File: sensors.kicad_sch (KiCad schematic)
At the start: 0 parts

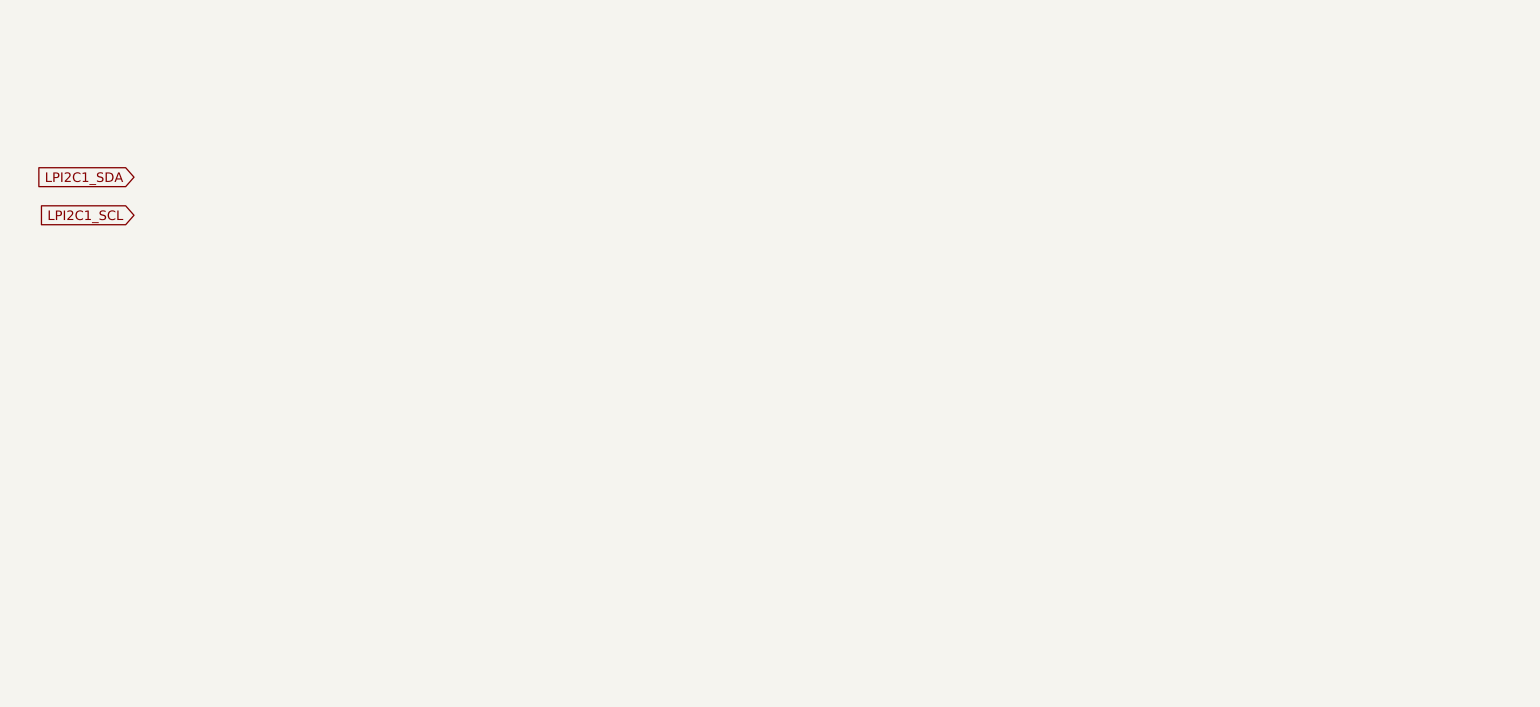
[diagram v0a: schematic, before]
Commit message: finished v1
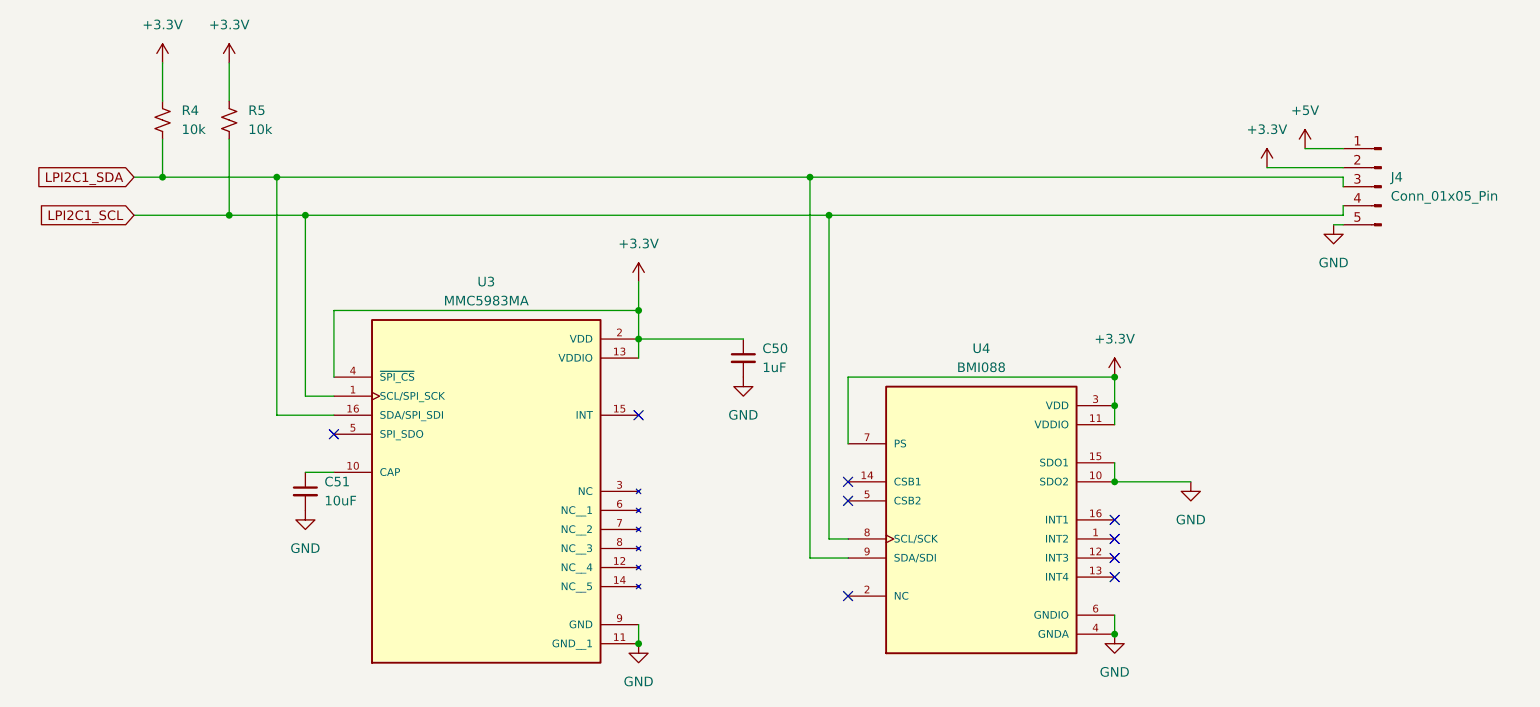
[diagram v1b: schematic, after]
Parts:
- added C50: 1uF, symbol Device:C_Small
- added C51: 10uF, symbol Device:C_Small
- added J4: Conn_01x05_Pin, symbol Connector:Conn_01x05_Pin
- added R4, R5: 10k, symbol Device:R_Small_US
- added U3: MMC5983MA, MMC5983MA:PQFN50P300X300X100-16N, symbol MMC5983MA:MMC5983MA
- added U4: BMI088, BMI088:PQFN50P450X300X100-16N, symbol BMI088:BMI088
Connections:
- net LPI2C1_SCL: now also J4.4 (Pin_4), R5.2, U3.1 (SCL/SPI_SCK), U4.8 (SCL/SCK)
- net LPI2C1_SDA: now also J4.3 (Pin_3), R4.2, U3.16 (SDA/SPI_SDI), U4.9 (SDA/SDI)
- new net: C51.1, U3.10 (CAP)
- new net +3.3V: C50.1, J4.2 (Pin_2), R4.1, R5.1, U3.13 (VDDIO), U3.2 (VDD), U3.4 (~{SPI_CS}), U4.11 (VDDIO), U4.3 (VDD), U4.7 (PS)
- new net +5V: J4.1 (Pin_1)
- new net GND: C50.2, C51.2, J4.5 (Pin_5), U3.11 (GND__1), U3.9 (GND), U4.10 (SDO2), U4.15 (SDO1), U4.4 (GNDA), U4.6 (GNDIO)
- no-connect marks 0 -> 9
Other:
- company: (none) -> Northeastern University
- title: (none) -> RT1050 DevBoard for Project Horizon
